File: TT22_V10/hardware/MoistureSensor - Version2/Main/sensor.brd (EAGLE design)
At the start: 45.7 x 46.7 mm, 10 parts

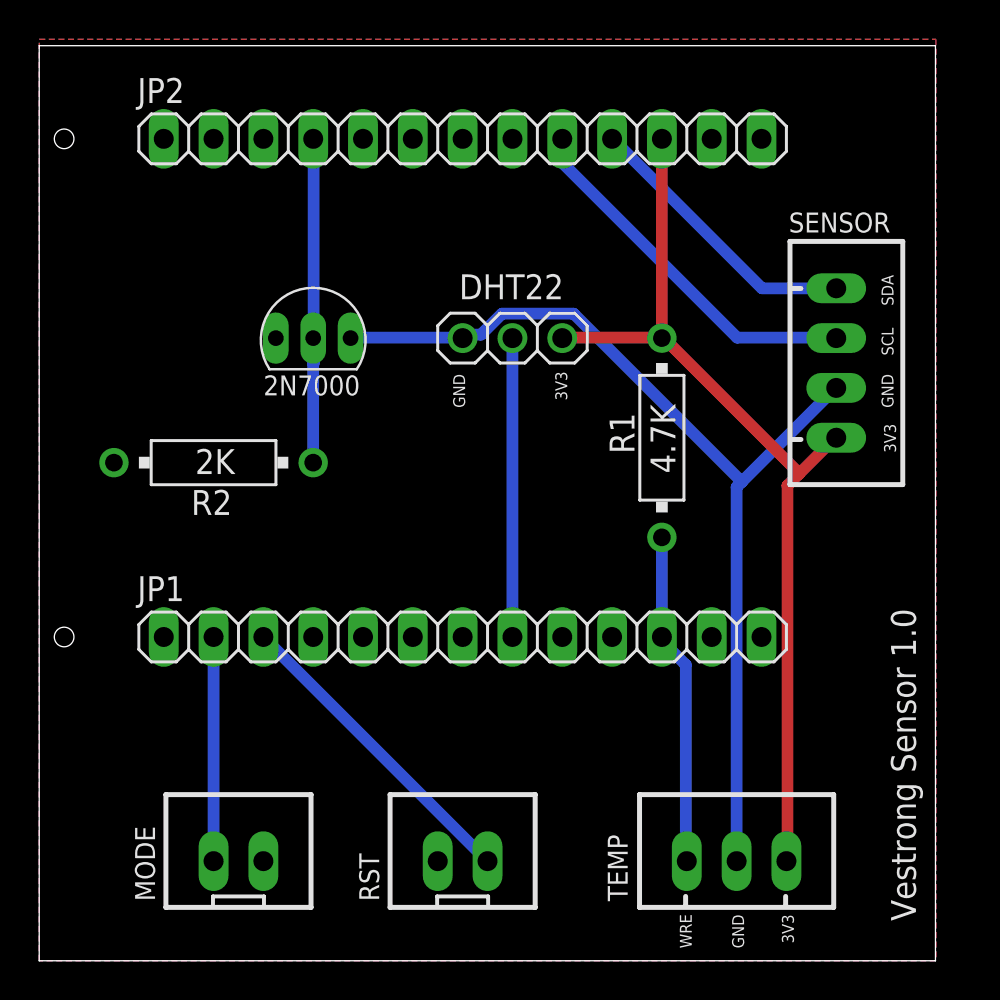
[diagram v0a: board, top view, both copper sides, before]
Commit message: reorg boards
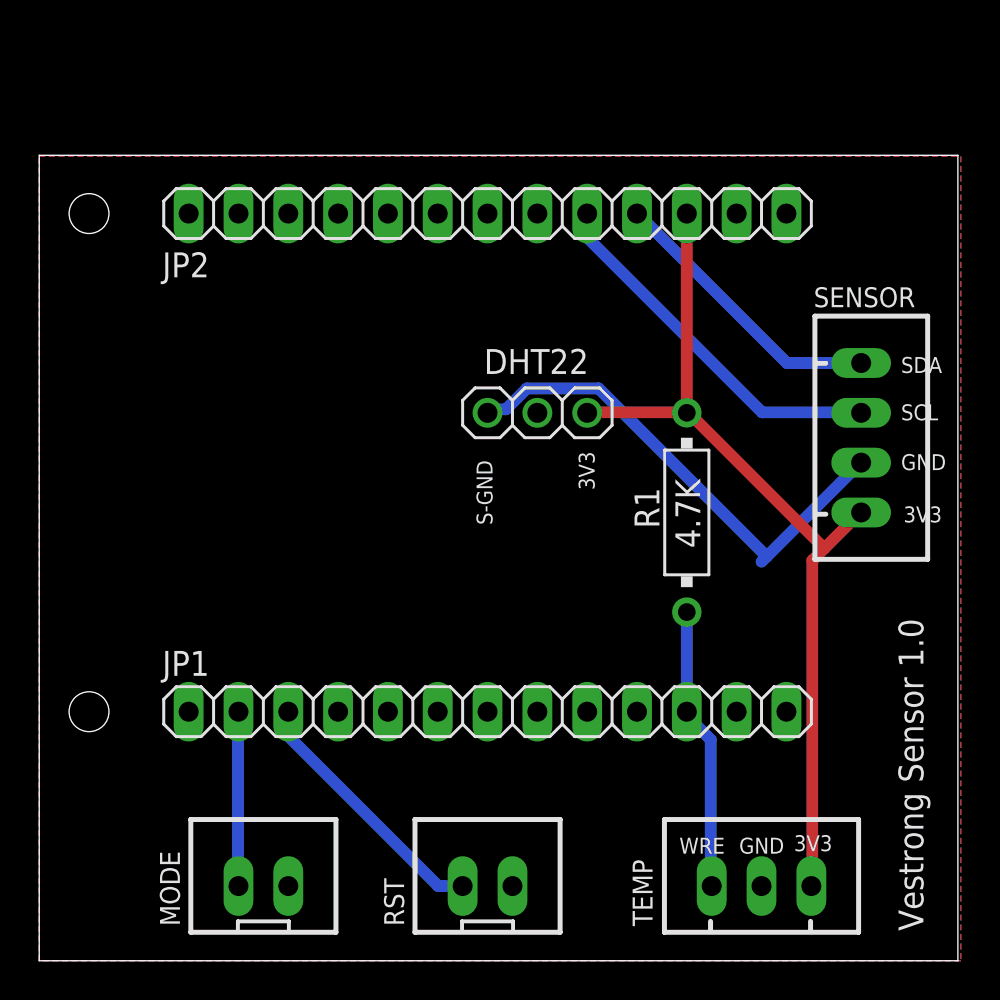
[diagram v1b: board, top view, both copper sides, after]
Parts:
- removed MOSFET1: 2N7000, 2N7000:TO92
- removed R2: 2K, resistor-power:HPS58
- moved R1 4.02 mm to (33.0, 22.9)
- moved JP1 4.02 mm to (22.9, 12.7)
- moved DHT22 4.02 mm to (25.4, 27.9)
- moved SENSOR 4.02 mm to (41.9, 26.7)
- moved JP2 4.02 mm to (22.9, 38.1)
- moved MODE 1.80 mm to (11.4, 3.81)
- moved RST 1.80 mm to (22.9, 3.81)
- moved TEMP 1.80 mm to (36.8, 3.81)
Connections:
- removed net DATA_T: DHT22.2, JP1.8
- removed net SENS_ENABLE: JP2.4, MOSFET1.B, R2.2
- new net N$2: DHT22.2, JP1.5
- net GND: now also DHT22.3, RST.2, TEMP.2; no longer MOSFET1.C, R2.1, RST.1
- net RST: now also RST.1; no longer RST.2
- net SENS_GND: no longer DHT22.3, MOSFET1.E, TEMP.2
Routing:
- net SENS_GND: track 50.3 -> 25.1 mm
- net SENS_ENABLE: track 16.6 -> 0.00 mm
- net DATA_T: track 15.2 -> 0.00 mm
- net RST: track 16.2 -> 13.3 mm
- net 1WIRE: track 17.0 -> 14.5 mm
- net 3.3V: track 47.8 -> 45.3 mm
- net MODE: track 11.4 -> 8.91 mm
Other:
- board size 45.7 x 46.7 mm -> 46.8 x 41.1 mm
- board text added: "S-GND"
